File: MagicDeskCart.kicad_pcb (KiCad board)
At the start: 2 copper layers, 7 parts, among them SW1 Reset, U1 74LS174, U2 74LS02, U3 27C020, U4 C64-Exp-Port

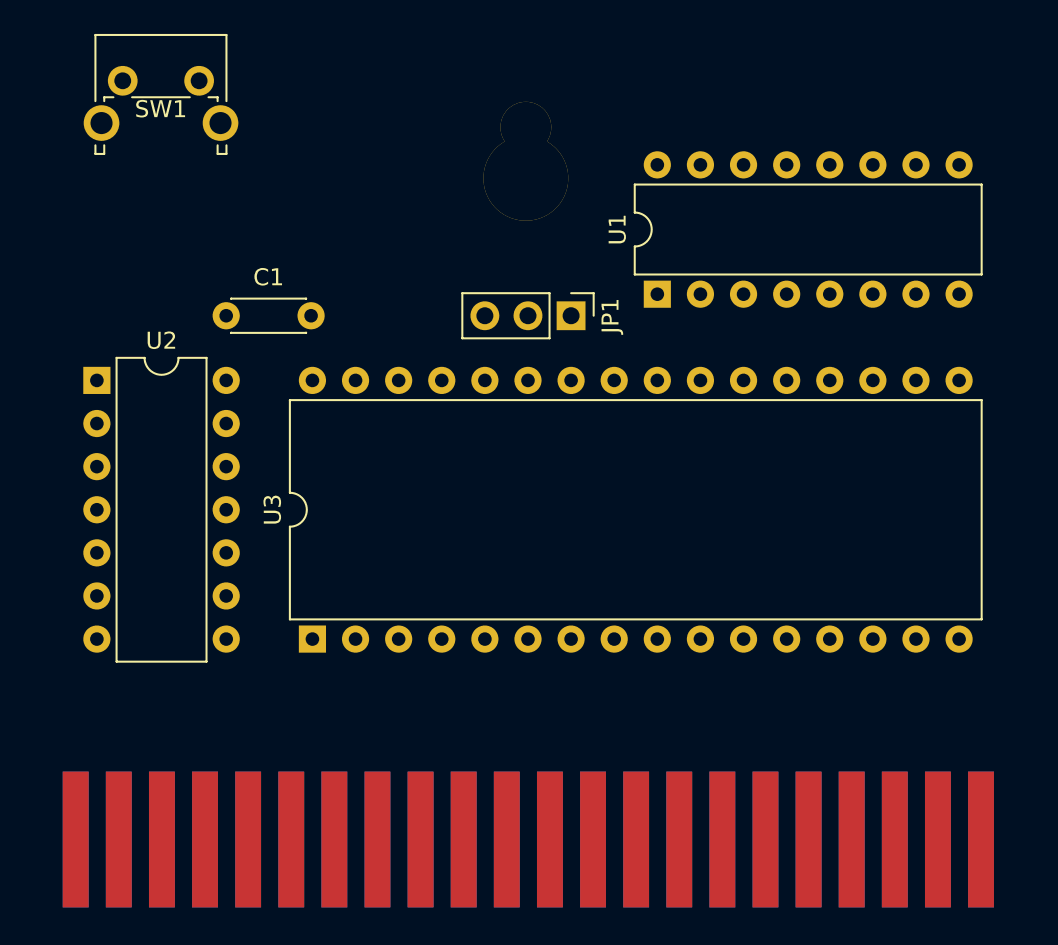
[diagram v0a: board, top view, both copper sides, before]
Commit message: Routing.
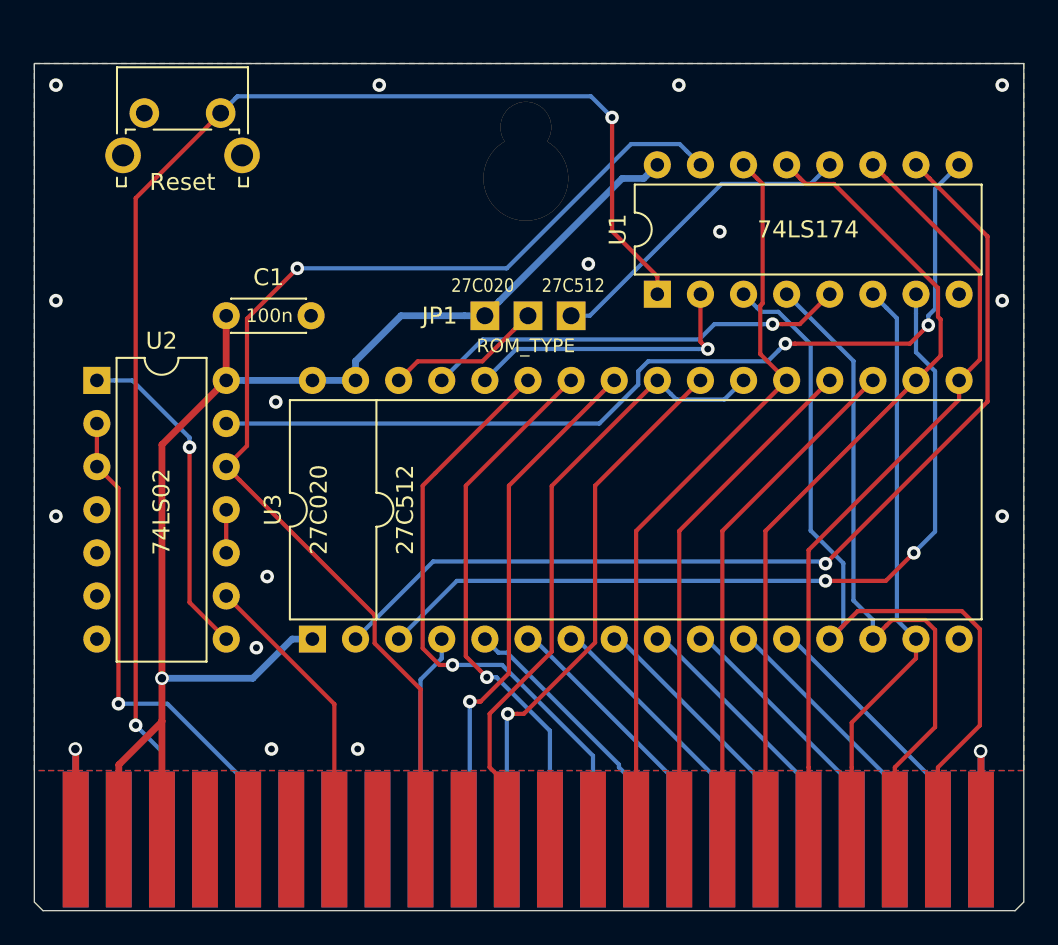
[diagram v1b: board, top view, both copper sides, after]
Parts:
- C1: value C -> 100n
- moved SW1 2.29 mm to (132.3, 57.0)
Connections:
- U4 pad 10: Net-(U4-Pad10) -> (no net)
- U4 pad 12: Net-(U4-Pad12) -> (no net)
- U4 pad 13: Net-(U4-Pad13) -> (no net)
- U4 pad 4: Net-(U4-Pad4) -> (no net)
- U4 pad 5: Net-(U4-Pad5) -> (no net)
- U4 pad 6: Net-(U4-Pad6) -> (no net)
- U4 pad 8: Net-(U4-Pad8) -> (no net)
- U4 pad B: Net-(U4-PadB) -> (no net)
- U4 pad D: Net-(U4-PadD) -> (no net)
- U4 pad F: Net-(U4-PadF) -> (no net)
- U4 pad H: Net-(U4-PadH) -> (no net)
- U4 pad J: Net-(U4-PadJ) -> (no net)
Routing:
- net +5V: track 0.00 -> 81.6 mm, vias 0 -> 1
- net Net-(SW1-Pad2): track 0.00 -> 81.0 mm, vias 0 -> 2
- net /DIS: track 0.00 -> 67.4 mm, vias 0 -> 1
- net /S16: track 0.00 -> 58.8 mm, vias 0 -> 1
- net /EN: track 0.00 -> 54.4 mm, vias 0 -> 2
- net /D4: track 0.00 -> 48.8 mm
- net /S15: track 0.00 -> 48.7 mm, vias 0 -> 2
- net /D0: track 0.00 -> 47.1 mm
- net /D3: track 0.00 -> 46.5 mm
- net /D7: track 0.00 -> 44.6 mm
- net /D1: track 0.00 -> 40.1 mm
- net Net-(U3-Pad22): track 0.00 -> 37.6 mm
- net /A8: track 0.00 -> 35.9 mm, vias 0 -> 1
- net /D2: track 0.00 -> 34.7 mm
- net /A10: track 0.00 -> 32.3 mm, vias 0 -> 1
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- added copper zone on B.Cu, net GND
- added copper zone on F.Cu, net GND
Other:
- board outline added: 58.3 x 49.9 mm
- net class Power added: clearance 0.3, trace_width 0.4, via_dia 0.8, via_drill 0.5
- board text added: "27C020"
- board text added: "27C512"
